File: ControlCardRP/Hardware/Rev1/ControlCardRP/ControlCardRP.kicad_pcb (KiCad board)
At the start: 4 copper layers, 53.5 x 49.5 mm, 153 parts, among them J1 Conn_02x20_Top_Bottom, J2 USB_C_Receptacle_USB2.0_16P, J3 SWD, J4 JST_PK BATTERY, J5 PIN_HEADER BATTERY, J8 ESP_IO, J9 Conn_01x03_Pin, Q1 NMOS, Q2 NMOS, SW1 SW_SPST, SW101 BOOT0, SW102 NRST, SW103 NRST, SW104 NRST, U1 AP33772SDKZ-xx-FA02, U102 RP2350B, U103 W25Q128JVS, U2 BQ24075RGT, U3 BQ27427YZFR, U4 MP28167GQ-A-P, U5 ESP32-C6-MINI-1, U6 AZ1117-3.3, U7 W25Q128JVP, Y1 12MHz

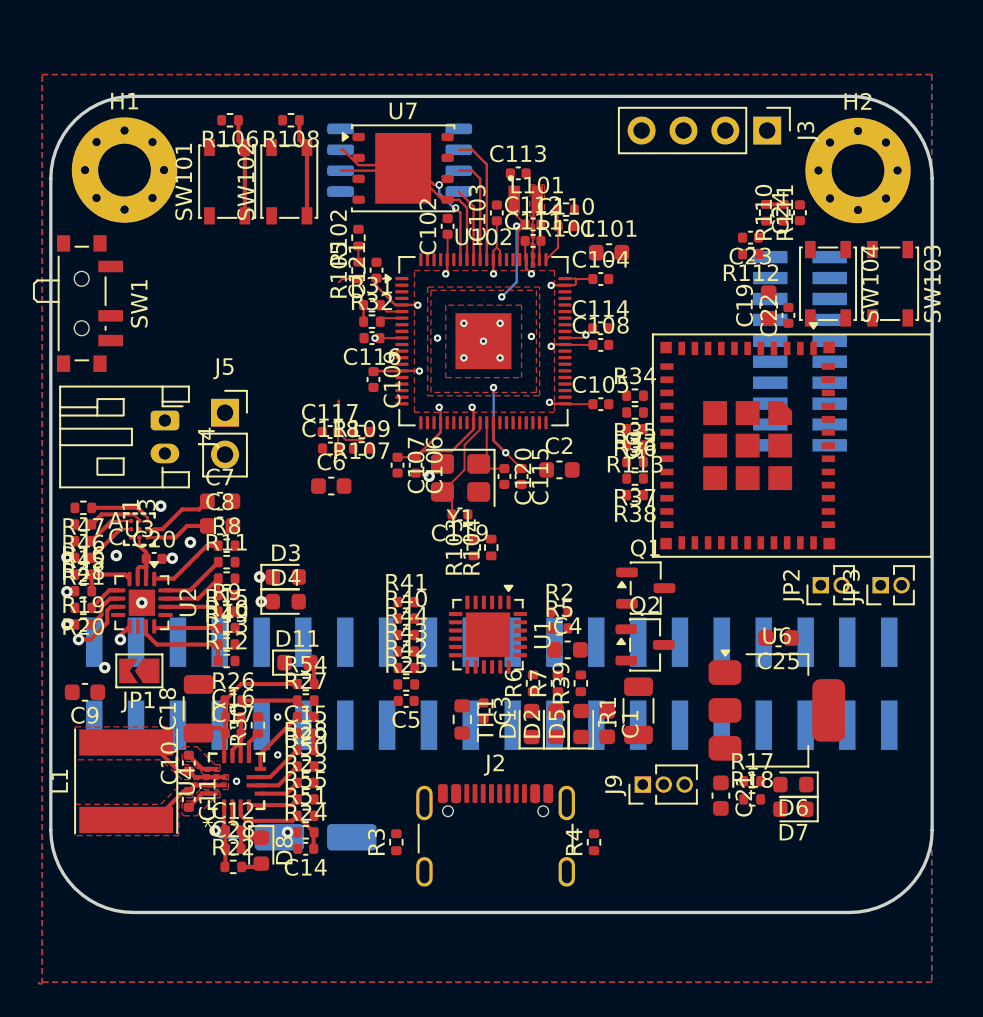
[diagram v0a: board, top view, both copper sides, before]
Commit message: A
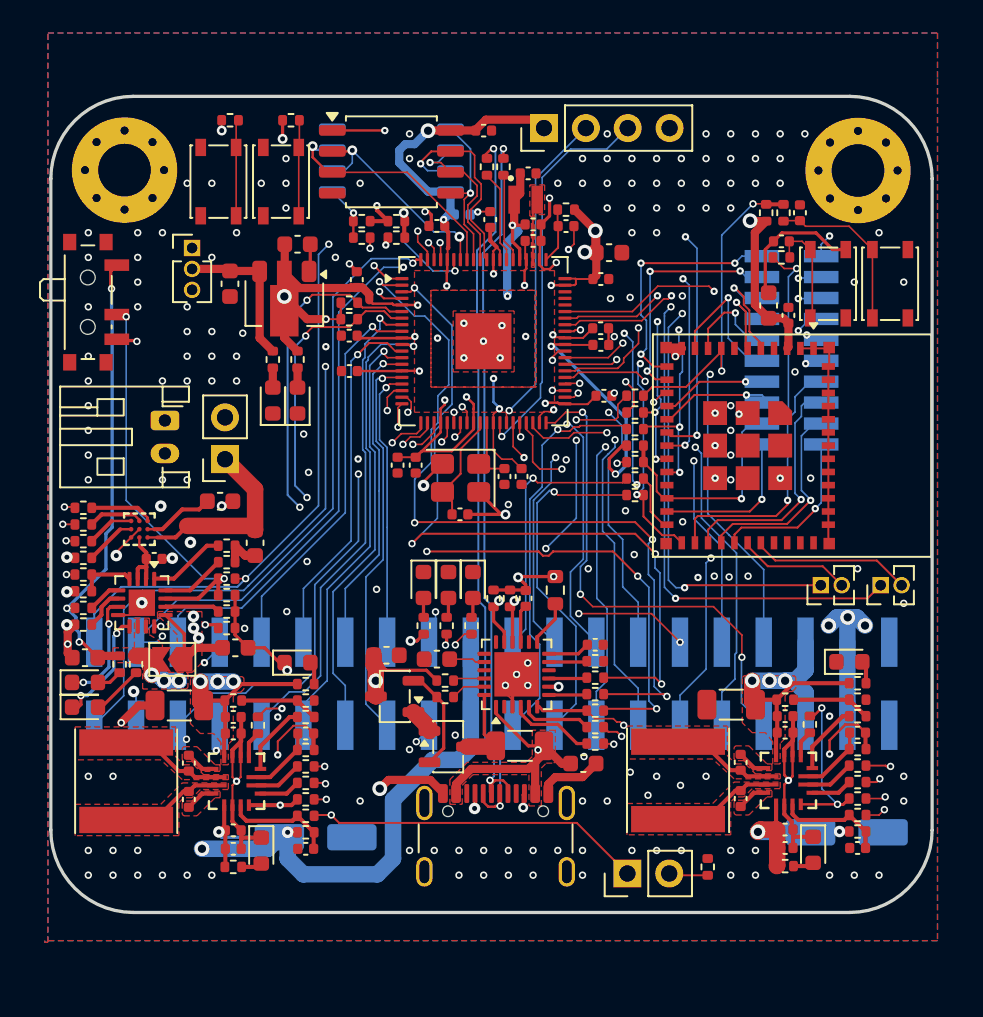
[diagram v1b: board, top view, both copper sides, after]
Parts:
- added C26: 100u, Capacitor_SMD:CP_Elec_5x5.4, B.Cu at (169.3, 109.2)
- added C27: 100n, Capacitor_SMD:C_0402_1005Metric, F.Cu at (165.6, 109.0)
- added C29: 10u, Capacitor_SMD:C_0402_1005Metric, F.Cu at (165.6, 110.1)
- added C30: 22n, Capacitor_SMD:C_0402_1005Metric, F.Cu at (170.0, 110.1)
- added C31: 100n, Capacitor_SMD:C_0402_1005Metric, F.Cu at (162.9, 107.1)
- added C32: 100n, Capacitor_SMD:C_0402_1005Metric, F.Cu at (162.9, 104.9)
- added C33: 100n, Capacitor_SMD:C_0402_1005Metric, F.Cu at (165.6, 102.1)
- added C34: 100n, Capacitor_SMD:C_0402_1005Metric, F.Cu at (165.6, 103.1)
- added C35: 100n, Capacitor_SMD:C_0402_1005Metric, F.Cu at (170.0, 103.1)
- added C36: 22u, Capacitor_SMD:C_1206_3216Metric, F.Cu at (162.3, 101.4)
- added D12: LED, LED_SMD:LED_0603_1608Metric, F.Cu at (169.5, 98.8)
- added D9: LED, LED_SMD:LED_0603_1608Metric, F.Cu at (167.3, 110.2)
- added J10: MAIN_POWER, Connector_PinHeader_2.54mm:PinHeader_1x02_P2.54mm_Vertical, F.Cu at (156.0, 111.7)
- added L2: 4u7, Inductor_SMD:L_Taiyo-Yuden_NR-60xx, F.Cu at (159.1, 106.0)
- added R52: 499k, Resistor_SMD:R_0402_1005Metric, F.Cu at (167.1, 102.6)
- added R53: 499k, Resistor_SMD:R_0402_1005Metric, F.Cu at (170.0, 109.1)
- added R56: 10k, Resistor_SMD:R_0402_1005Metric, F.Cu at (165.6, 111.2)
- added R57: 0R, Resistor_SMD:R_0402_1005Metric, F.Cu at (170.0, 106.1)
- added R58: 0R, Resistor_SMD:R_0402_1005Metric, F.Cu at (170.0, 105.1)
- added R59: 0R, Resistor_SMD:R_0402_1005Metric, F.Cu at (170.0, 108.1)
- added R60: 0R, Resistor_SMD:R_0402_1005Metric, F.Cu at (170.0, 107.1)
- added R61: 430k, Resistor_SMD:R_0402_1005Metric, F.Cu at (165.6, 101.1)
- added R62: 107k, Resistor_SMD:R_0402_1005Metric, F.Cu at (170.0, 101.1)
- added R63: 806k, Resistor_SMD:R_0402_1005Metric, F.Cu at (170.0, 102.1)
- added R64: 499k, Resistor_SMD:R_0402_1005Metric, F.Cu at (170.0, 104.1)
- added R65: 10k, Resistor_SMD:R_0402_1005Metric, F.Cu at (170.0, 100.1)
- added R66: 10k, Resistor_SMD:R_0402_1005Metric, F.Cu at (160.9, 111.3)
- added U8: MP28167GQ-A-P, footprints:QFN-16_MP28167_MNP, F.Cu at (165.8, 106.0)
- C117: moved to B.Cu
- SW1: value SW_SPST -> SW_SPDT
- U6: footprint Package_TO_SOT_SMD:SOT-223-3_TabPin2 -> Package_TO_SOT_SMD:SOT-89-3
- U7: value W25Q128JVP -> W25Q128JVS; footprint Package_SON:WSON-8-1EP_6x5mm_P1.27mm_EP3.4x4.3mm -> Package_SO:SOIC-8_5.3x5.3mm_P1.27mm
- moved C21 43.1 mm to (131.9, 75.9)
- moved J9 42.5 mm to (129.6, 73.7), turned to 0 degrees
- moved D6 39.3 mm to (134.5, 83.0), turned to 90 degrees
- moved D7 39.0 mm to (136.0, 83.0), turned to 90 degrees
- moved U6 38.8 mm to (135.2, 77.1), turned to -90 degrees
- moved R17 38.8 mm to (134.5, 80.5), turned to -90 degrees
- moved R18 38.4 mm to (136.0, 80.5), turned to -90 degrees
- moved C25 37.7 mm to (136.0, 73.5), turned to 0 degrees
- moved R103 23.2 mm to (148.5, 68.8), turned to -90 degrees
- moved R104 23.1 mm to (147.5, 68.8), turned to -90 degrees
- moved C118 21.4 mm to (147.3, 66.6), turned to 180 degrees
- moved Q1 16.6 mm to (141.9, 100.9), turned to 180 degrees
- moved R3 15.9 mm to (147.9, 95.0), turned to -90 degrees
- moved R4 15.7 mm to (148.9, 95.0), turned to -90 degrees
- moved C117 15.4 mm to (146.0, 71.7), turned to 180 degrees
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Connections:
- net /Controller/GPIO45/ADC5 renamed /GPIO45
- net /Controller/GPIO46/ADC6 renamed /GPIO46
- net /Controller/GPIO47/ADC7 renamed /GPIO47
- net Net-(U102-USB_DM) renamed /Controller/USB_DN
- C16 pad 1: /Power 5V/OUT -> +5V
- C17 pad 1: /Power 5V/OUT -> +5V
- C18 pad 1: /Power 5V/OUT -> +5V
- C8 pad 1: Net-(J4-Pin_1) -> Net-(J4-Pin_2)
- J1 pad 1: /GPIO0 -> /GPIO40
- J1 pad 17: /GPIO18 -> /GPIO34
- J1 pad 18: /GPIO19 -> /GPIO35
- J1 pad 3: /GPIO2 -> /GPIO41
- J1 pad 35: /GPIO34 -> /POWER_AUX
- J1 pad 36: /GPIO35 -> /POWER_AUX
- J1 pad 6: /GPIO5 -> /GPIO42
- J1 pad 7: /GPIO6 -> /GPIO43
- J1 pad 8: /GPIO7 -> /GPIO44
- J2 pad A6: Net-(U1-DP) -> /USB_D+
- J2 pad A7: Net-(U1-DN) -> /USB_D-
- J2 pad B6: Net-(U1-DP) -> /USB_D+
- J2 pad B7: Net-(U1-DN) -> /USB_D-
- J4 pad 1: Net-(J4-Pin_1) -> GND
- J4 pad 2: GND -> Net-(J4-Pin_2)
- J5 pad 1: Net-(J4-Pin_1) -> Net-(J4-Pin_2)
- R103 pad 1: /Controller/USB_DM -> /USB_D-
- R104 pad 1: /Controller/USB_DP -> /USB_D+
- R104 pad 2: Net-(U102-USB_DP) -> /Controller/USB_DP
- R26 pad 1: /Power 5V/OUT -> +5V
- R44 pad 2: Net-(U1-FLIP) -> /USB-C PD/FLIP
- R51 pad 2: /GPIO4 -> /Power 5V/POWER_EN
- R54 pad 1: /Power 5V/OUT -> +5V
- R55 pad 2: /Power 5V/POWER_ALT -> /GPIO4
- SW1 pad 1: /Battery Management/SYSOFF -> /BATT_OUT
- SW1 pad 2: /BATT_OUT -> /Battery Management/SYSOFF
- SW1 pad 3: (no net) -> GND
- U1 pad 18: Net-(U1-DN) -> unconnected-(U1-DN-Pad18)
- U1 pad 19: Net-(U1-DP) -> unconnected-(U1-DP-Pad19)
- U1 pad 6: Net-(U1-FLIP) -> /USB-C PD/FLIP
- U102 pad 49: /Controller/GPIO40/ADC0 -> /GPIO40
- U102 pad 52: /Controller/GPIO41/ADC1 -> /GPIO41
- U102 pad 53: /Controller/GPIO42/ADC2 -> /GPIO42
- U102 pad 54: /Controller/GPIO43/ADC3 -> /GPIO43
- U102 pad 55: /Controller/GPIO44/ADC4 -> /GPIO44
- U102 pad 67: Net-(U102-USB_DP) -> /Controller/USB_DP
- U3 pad C3: Net-(J4-Pin_1) -> Net-(J4-Pin_2)
- U4 pad 12: /Power 5V/OUT -> +5V
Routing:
- net +3V3: track 40.5 -> 173.7 mm, vias 10 -> 19
- net /BATT_OUT: track 15.8 -> 127.9 mm, vias 2 -> 11
- net GND: track 14.7 -> 118.8 mm, vias 18 -> 185
- net /GPIO13: track 0.00 -> 73.1 mm, vias 0 -> 3
- net /GPIO9: track 1.40 -> 72.9 mm, vias 0 -> 5
- net /GPIO12: track 0.00 -> 71.2 mm, vias 0 -> 3
- net /GPIO8: track 1.47 -> 71.8 mm, vias 0 -> 5
- net /GPIO44: track 0.00 -> 63.2 mm, vias 0 -> 3
- net /GPIO10: track 0.00 -> 56.9 mm, vias 0 -> 3
- net /GPIO42: track 0.00 -> 56.7 mm, vias 0 -> 2
- net /GPIO43: track 0.00 -> 56.5 mm, vias 0 -> 3
- net /USB_D+: track 0.00 -> 55.1 mm, vias 0 -> 2
- net /USB_D-: track 0.00 -> 55.1 mm, vias 0 -> 2
- net /GPIO41: track 0.00 -> 54.5 mm, vias 0 -> 3
- net /GPIO11: track 0.00 -> 52.0 mm, vias 0 -> 3
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- added copper zone on F.Cu, net +5V
- added copper zone on In2.Cu, net +5V
- added copper zone on F.Cu, net /BATT_OUT
- added copper zone on In1.Cu, net /BATT_OUT
- added copper zone on F.Cu, net /POWER_AUX
- added copper zone on F.Cu, net /USB-C PD/VBUS
- added copper zone on F.Cu, net Net-(U8-BST1)
- added copper zone on F.Cu, net Net-(U8-BST2)
- added copper zone on F.Cu, net Net-(U8-SW1)
- added copper zone on F.Cu, net Net-(U8-SW2)
- added copper zone on F.Cu, net VBUS_UCPD
